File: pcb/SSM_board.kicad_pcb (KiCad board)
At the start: 4 copper layers, 100 x 100 mm, 184 parts, among them IC1 STPIC6C595TTR, IC2 STPIC6C595TTR, IC3 STPIC6C595TTR, IC4 STPIC6C595TTR, IC5 STPIC6C595TTR, IC6 STPIC6C595TTR, IC7 STPIC6C595TTR, IC8 STPIC6C595TTR, J1 DA15_Pins_MountingHoles, J2 DA15_Pins_MountingHoles, U101 GAQY212GS, U102 GAQY212GS, U103 GAQY212GS, U104 GAQY212GS, U105 GAQY212GS, U106 GAQY212GS, U107 GAQY212GS, U108 GAQY212GS, U201 GAQY212GS, U202 GAQY212GS, U203 GAQY212GS, U204 GAQY212GS, U205 GAQY212GS, U206 GAQY212GS, U207 GAQY212GS, U208 GAQY212GS, U301 GAQY212GS, U302 GAQY212GS, U303 GAQY212GS, U304 GAQY212GS, U305 GAQY212GS, U306 GAQY212GS, U307 GAQY212GS, U308 GAQY212GS, U401 GAQY212GS, U402 GAQY212GS, U403 GAQY212GS, U404 GAQY212GS, U405 GAQY212GS, U406 GAQY212GS, U407 GAQY212GS, U408 GAQY212GS, U501 GAQY212GS, U502 GAQY212GS, U503 GAQY212GS, U504 GAQY212GS, U505 GAQY212GS, U506 GAQY212GS, U507 GAQY212GS, U508 GAQY212GS, U601 GAQY212GS, U602 GAQY212GS, U603 GAQY212GS, U604 GAQY212GS, U605 GAQY212GS, U606 GAQY212GS, U607 GAQY212GS, U608 GAQY212GS, U609 GAQY212GS, U610 GAQY212GS, U611 GAQY212GS, U612 GAQY212GS, U701 GAQY212GS, U702 GAQY212GS, U703 GAQY212GS, U704 GAQY212GS, U705 GAQY212GS, U706 GAQY212GS, U707 GAQY212GS, U708 GAQY212GS, U709 GAQY212GS, U710 GAQY212GS, U711 GAQY212GS, U712 GAQY212GS

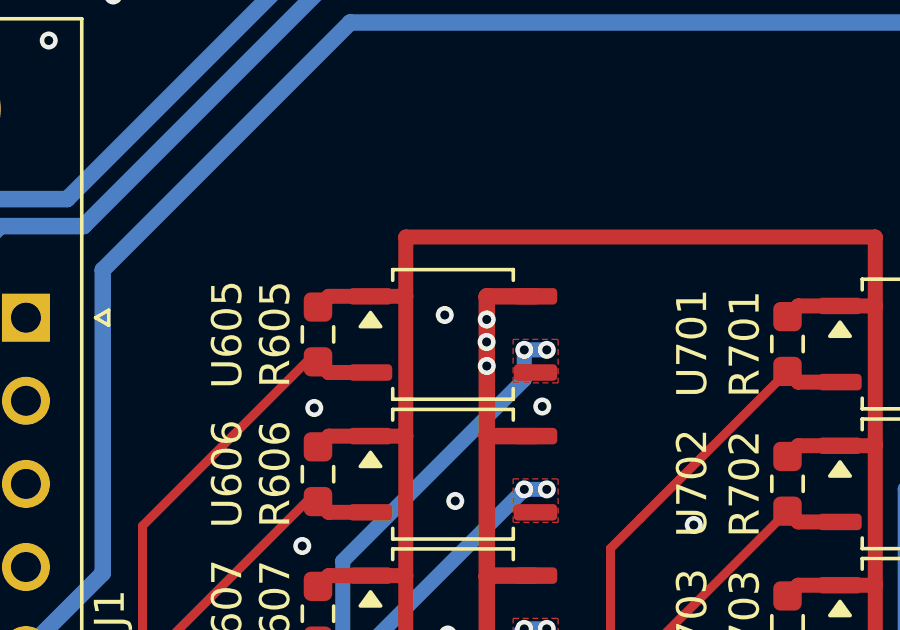
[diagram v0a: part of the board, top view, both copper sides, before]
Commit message: Ready for production
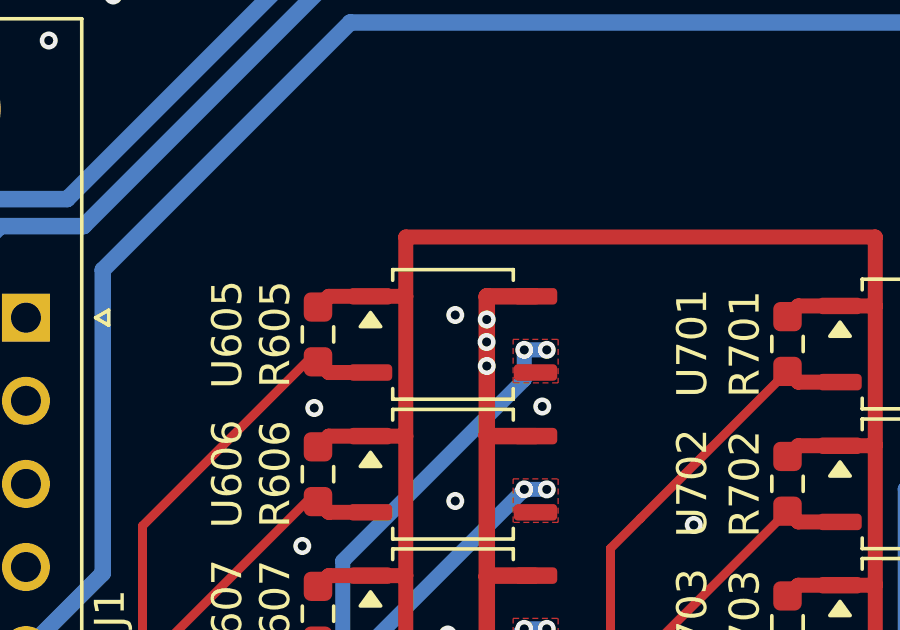
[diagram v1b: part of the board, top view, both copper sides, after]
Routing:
- net Net-(J1-Pad2): track 147.6 -> 149.0 mm
- net Net-(J1-Pad7): track 165.9 -> 167.2 mm
- net Net-(J1-Pad6): track 166.6 -> 168.0 mm
- net Net-(J1-Pad3): track 128.5 -> 129.9 mm
- net Net-(J1-P9): track 138.3 -> 139.6 mm
- net Net-(J1-Pad8): track 162.5 -> 163.8 mm
- net Net-(J1-Pad4): track 106.5 -> 107.9 mm
- net Net-(J1-Pad1): track 164.1 -> 165.5 mm
- net Net-(J1-P12): track 139.3 -> 140.6 mm
